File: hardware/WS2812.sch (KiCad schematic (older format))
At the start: 39 parts, among them J2 WS2812_HEADER, U3 74AHCT1G125

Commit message: update footprint,
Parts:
- D10, D11, D12, D13, D14, D15, D16, D17, D18, D19, D20, D21, D22, D23, D6, D7, D8, D9: footprint LED_SMD:LED_WS2812B_PLCC4_5.0x5.0mm_P3.2mm -> footprint-lib:LED_WS2812B_5050_white
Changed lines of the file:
@@
 EESchema Schematic File Version 4
-LIBS:stm32_aux_keyboard-cache
 EELAYER 29 0
 EELAYER END
 $Descr A4 11693 8268
 encoding utf-8
-Sheet 5 13
+Sheet 1 1
 Title ""
 Date ""
@@
 F 0 "D6" H 4100 2550 50  0000 L CNN
 F 1 "WS2812B" H 4100 2500 50  0000 L CNN
-F 2 "LED_SMD:LED_WS2812B_PLCC4_5.0x5.0mm_P3.2mm" H 3800 2200 50  0001 L TNN
+F 2 "footprint-lib:LED_WS2812B_5050_white" H 3800 2200 50  0001 L TNN
 F 3 "https://cdn-shop.adafruit.com/datasheets/WS2812B.pdf" H 3850 2125 50  0001 L TNN
 	1    3750 2500
@@
 F 0 "D7" H 5100 2550 50  0000 L CNN
 F 1 "WS2812B" H 5100 2500 50  0000 L CNN
-F 2 "LED_SMD:LED_WS2812B_PLCC4_5.0x5.0mm_P3.2mm" H 4800 2200 50  0001 L TNN
+F 2 "footprint-lib:LED_WS2812B_5050_white" H 4800 2200 50  0001 L TNN
 F 3 "https://cdn-shop.adafruit.com/datasheets/WS2812B.pdf" H 4850 2125 50  0001 L TNN
 	1    4750 2500
@@
 F 0 "D8" H 6100 2550 50  0000 L CNN
 F 1 "WS2812B" H 6100 2500 50  0000 L CNN
-F 2 "LED_SMD:LED_WS2812B_PLCC4_5.0x5.0mm_P3.2mm" H 5800 2200 50  0001 L TNN
+F 2 "footprint-lib:LED_WS2812B_5050_white" H 5800 2200 50  0001 L TNN
 F 3 "https://cdn-shop.adafruit.com/datasheets/WS2812B.pdf" H 5850 2125 50  0001 L TNN
 	1    5750 2500
@@
 F 0 "D9" H 7100 2550 50  0000 L CNN
 F 1 "WS2812B" H 7100 2500 50  0000 L CNN
-F 2 "LED_SMD:LED_WS2812B_PLCC4_5.0x5.0mm_P3.2mm" H 6800 2200 50  0001 L TNN
+F 2 "footprint-lib:LED_WS2812B_5050_white" H 6800 2200 50  0001 L TNN
 F 3 "https://cdn-shop.adafruit.com/datasheets/WS2812B.pdf" H 6850 2125 50  0001 L TNN
 	1    6750 2500
@@
 F 0 "D10" H 8100 2550 50  0000 L CNN
 F 1 "WS2812B" H 8100 2500 50  0000 L CNN
-F 2 "LED_SMD:LED_WS2812B_PLCC4_5.0x5.0mm_P3.2mm" H 7800 2200 50  0001 L TNN
+F 2 "footprint-lib:LED_WS2812B_5050_white" H 7800 2200 50  0001 L TNN
 F 3 "https://cdn-shop.adafruit.com/datasheets/WS2812B.pdf" H 7850 2125 50  0001 L TNN
 	1    7750 2500
@@
 F 0 "D11" H 9100 2550 50  0000 L CNN
 F 1 "WS2812B" H 9100 2500 50  0000 L CNN
-F 2 "LED_SMD:LED_WS2812B_PLCC4_5.0x5.0mm_P3.2mm" H 8800 2200 50  0001 L TNN
+F 2 "footprint-lib:LED_WS2812B_5050_white" H 8800 2200 50  0001 L TNN
 F 3 "https://cdn-shop.adafruit.com/datasheets/WS2812B.pdf" H 8850 2125 50  0001 L TNN
 	1    8750 2500
@@
 F 0 "D12" H 4100 4150 50  0000 L CNN
 F 1 "WS2812B" H 4100 4100 50  0000 L CNN
-F 2 "LED_SMD:LED_WS2812B_PLCC4_5.0x5.0mm_P3.2mm" H 3800 3800 50  0001 L TNN
+F 2 "footprint-lib:LED_WS2812B_5050_white" H 3800 3800 50  0001 L TNN
 F 3 "https://cdn-shop.adafruit.com/datasheets/WS2812B.pdf" H 3850 3725 50  0001 L TNN
 	1    3750 4100
@@
 F 0 "D13" H 5100 4150 50  0000 L CNN
 F 1 "WS2812B" H 5100 4100 50  0000 L CNN
-F 2 "LED_SMD:LED_WS2812B_PLCC4_5.0x5.0mm_P3.2mm" H 4800 3800 50  0001 L TNN
+F 2 "footprint-lib:LED_WS2812B_5050_white" H 4800 3800 50  0001 L TNN
 F 3 "https://cdn-shop.adafruit.com/datasheets/WS2812B.pdf" H 4850 3725 50  0001 L TNN
 	1    4750 4100
@@
 F 0 "D14" H 6100 4150 50  0000 L CNN
 F 1 "WS2812B" H 6100 4100 50  0000 L CNN
-F 2 "LED_SMD:LED_WS2812B_PLCC4_5.0x5.0mm_P3.2mm" H 5800 3800 50  0001 L TNN
+F 2 "footprint-lib:LED_WS2812B_5050_white" H 5800 3800 50  0001 L TNN
 F 3 "https://cdn-shop.adafruit.com/datasheets/WS2812B.pdf" H 5850 3725 50  0001 L TNN
 	1    5750 4100
@@
 F 0 "D15" H 7100 4150 50  0000 L CNN
 F 1 "WS2812B" H 7100 4100 50  0000 L CNN
-F 2 "LED_SMD:LED_WS2812B_PLCC4_5.0x5.0mm_P3.2mm" H 6800 3800 50  0001 L TNN
+F 2 "footprint-lib:LED_WS2812B_5050_white" H 6800 3800 50  0001 L TNN
 F 3 "https://cdn-shop.adafruit.com/datasheets/WS2812B.pdf" H 6850 3725 50  0001 L TNN
 	1    6750 4100
@@
 F 0 "D16" H 8100 4150 50  0000 L CNN
 F 1 "WS2812B" H 8100 4100 50  0000 L CNN
-F 2 "LED_SMD:LED_WS2812B_PLCC4_5.0x5.0mm_P3.2mm" H 7800 3800 50  0001 L TNN
+F 2 "footprint-lib:LED_WS2812B_5050_white" H 7800 3800 50  0001 L TNN
 F 3 "https://cdn-shop.adafruit.com/datasheets/WS2812B.pdf" H 7850 3725 50  0001 L TNN
 	1    7750 4100
@@
 F 0 "D17" H 9100 4150 50  0000 L CNN
 F 1 "WS2812B" H 9100 4100 50  0000 L CNN
-F 2 "LED_SMD:LED_WS2812B_PLCC4_5.0x5.0mm_P3.2mm" H 8800 3800 50  0001 L TNN
+F 2 "footprint-lib:LED_WS2812B_5050_white" H 8800 3800 50  0001 L TNN
 F 3 "https://cdn-shop.adafruit.com/datasheets/WS2812B.pdf" H 8850 3725 50  0001 L TNN
 	1    8750 4100
@@
 F 0 "D18" H 4100 5650 50  0000 L CNN
 F 1 "WS2812B" H 4100 5600 50  0000 L CNN
-F 2 "LED_SMD:LED_WS2812B_PLCC4_5.0x5.0mm_P3.2mm" H 3800 5300 50  0001 L TNN
+F 2 "footprint-lib:LED_WS2812B_5050_white" H 3800 5300 50  0001 L TNN
 F 3 "https://cdn-shop.adafruit.com/datasheets/WS2812B.pdf" H 3850 5225 50  0001 L TNN
 	1    3750 5600
@@
 F 0 "D19" H 5100 5650 50  0000 L CNN
 F 1 "WS2812B" H 5100 5600 50  0000 L CNN
-F 2 "LED_SMD:LED_WS2812B_PLCC4_5.0x5.0mm_P3.2mm" H 4800 5300 50  0001 L TNN
+F 2 "footprint-lib:LED_WS2812B_5050_white" H 4800 5300 50  0001 L TNN
 F 3 "https://cdn-shop.adafruit.com/datasheets/WS2812B.pdf" H 4850 5225 50  0001 L TNN
 	1    4750 5600
@@
 F 0 "D20" H 6100 5650 50  0000 L CNN
 F 1 "WS2812B" H 6100 5600 50  0000 L CNN
-F 2 "LED_SMD:LED_WS2812B_PLCC4_5.0x5.0mm_P3.2mm" H 5800 5300 50  0001 L TNN
+F 2 "footprint-lib:LED_WS2812B_5050_white" H 5800 5300 50  0001 L TNN
 F 3 "https://cdn-shop.adafruit.com/datasheets/WS2812B.pdf" H 5850 5225 50  0001 L TNN
 	1    5750 5600
@@
 F 0 "D21" H 7100 5650 50  0000 L CNN
 F 1 "WS2812B" H 7100 5600 50  0000 L CNN
-F 2 "LED_SMD:LED_WS2812B_PLCC4_5.0x5.0mm_P3.2mm" H 6800 5300 50  0001 L TNN
+F 2 "footprint-lib:LED_WS2812B_5050_white" H 6800 5300 50  0001 L TNN
 F 3 "https://cdn-shop.adafruit.com/datasheets/WS2812B.pdf" H 6850 5225 50  0001 L TNN
 	1    6750 5600
@@
 F 0 "D22" H 8100 5650 50  0000 L CNN
 F 1 "WS2812B" H 8100 5600 50  0000 L CNN
-F 2 "LED_SMD:LED_WS2812B_PLCC4_5.0x5.0mm_P3.2mm" H 7800 5300 50  0001 L TNN
+F 2 "footprint-lib:LED_WS2812B_5050_white" H 7800 5300 50  0001 L TNN
 F 3 "https://cdn-shop.adafruit.com/datasheets/WS2812B.pdf" H 7850 5225 50  0001 L TNN
 	1    7750 5600
@@
 F 0 "D23" H 9100 5650 50  0000 L CNN
 F 1 "WS2812B" H 9100 5600 50  0000 L CNN
-F 2 "LED_SMD:LED_WS2812B_PLCC4_5.0x5.0mm_P3.2mm" H 8800 5300 50  0001 L TNN
+F 2 "footprint-lib:LED_WS2812B_5050_white" H 8800 5300 50  0001 L TNN
 F 3 "https://cdn-shop.adafruit.com/datasheets/WS2812B.pdf" H 8850 5225 50  0001 L TNN
 	1    8750 5600

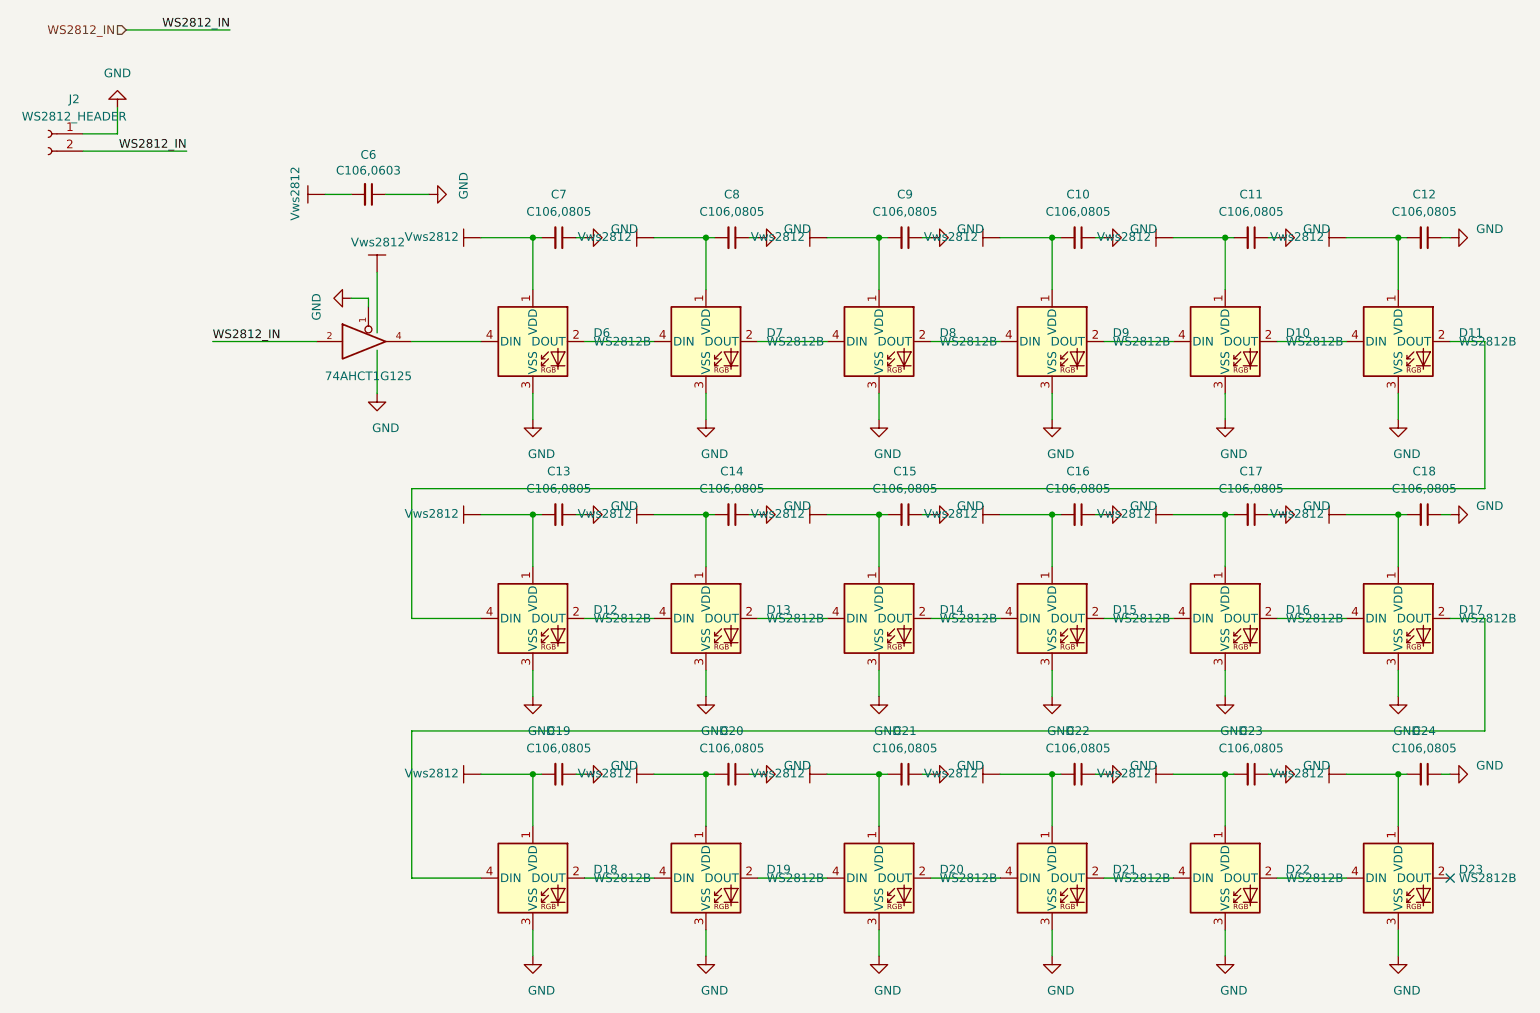
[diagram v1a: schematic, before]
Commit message: update route,
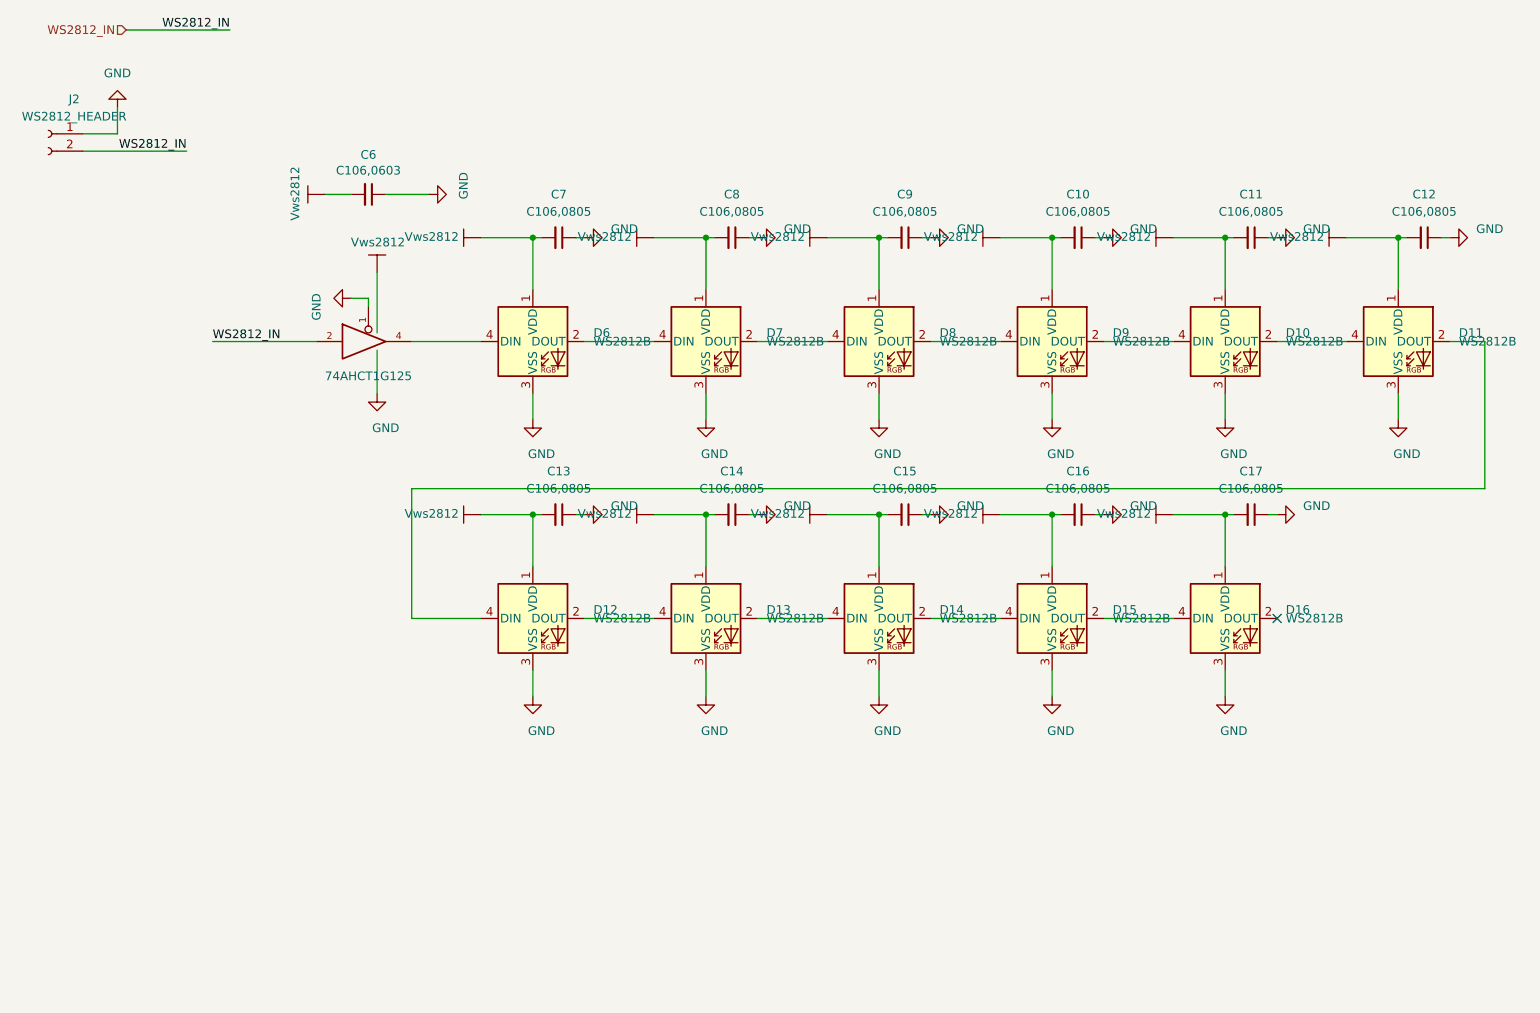
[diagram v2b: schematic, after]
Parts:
- removed C18, C19, C20, C21, C22, C23, C24: C106,0805, Capacitor_SMD:C_0805_2012Metric_Pad1.15x1.40mm_HandSolder, symbol taobao-c:C106,0805
- removed D17, D18, D19, D20, D21, D22, D23: WS2812B, footprint-lib:LED_WS2812B_5050_white, symbol LED:WS2812B
